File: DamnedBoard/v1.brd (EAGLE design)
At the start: 49.3 x 16.5 mm, 20 parts, among them J1 CORTEX_DEBUG_SMD, J2 GND, U1 EFM32ZG108, U2 MAX44009EDT+T21-0490D-M

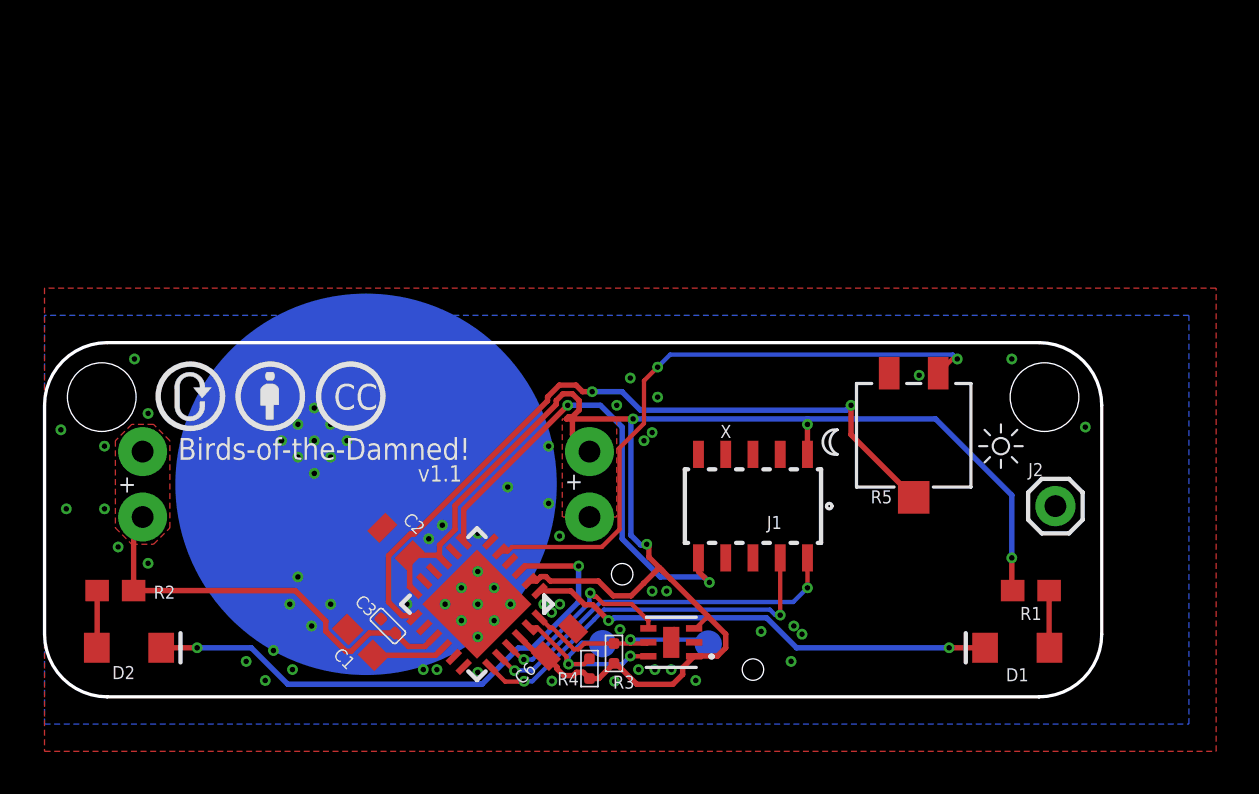
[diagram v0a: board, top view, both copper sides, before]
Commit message: Adding scheatic png
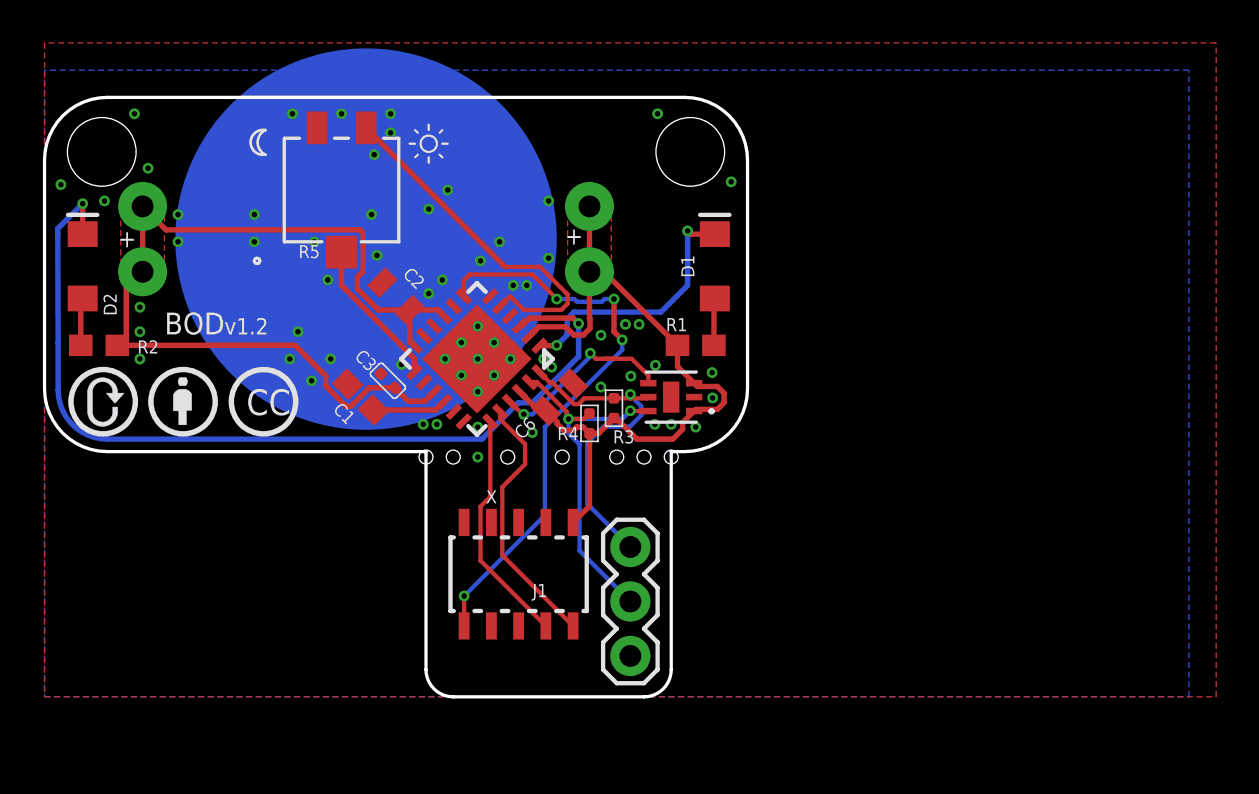
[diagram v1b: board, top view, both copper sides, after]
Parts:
- removed TP1, TP2: TEST-POINT3X5, SparkFun-Connectors:PAD.03X.05
- J2: value GND -> debug; device SparkFun-Connectors:1X01 -> SparkFun-Connectors:1X03
- moved R5 29.0 mm to (13.8, 23.6)
- moved D1 22.7 mm to (31.2, 20.1), turned to 90 degrees
- moved J2 19.9 mm to (27.3, 6.99), turned to 270 degrees
- moved R1 19.4 mm to (30.4, 16.4)
- moved D2 17.9 mm to (1.78, 20.1), turned to 90 degrees
- moved U$2 14.0 mm to (30.6, 11.9)
- moved R2 11.5 mm to (2.54, 16.4)
- moved C1 11.4 mm to (14.7, 14.0)
- moved C2 11.4 mm to (16.4, 18.7)
- moved C3 11.4 mm to (16.0, 14.7)
- moved C6 11.4 mm to (24.0, 14.0)
- moved G1 11.4 mm to (25.4, 22.9)
- moved R3 11.4 mm to (25.4, 12.7)
- moved R4 11.4 mm to (26.5, 13.5)
- moved U1 11.4 mm to (23.7, 15.7)
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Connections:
- net SCL: now also J2.1; no longer TP2.P$1
- net SDA: now also J2.2; no longer TP1.P$1
- net VSS: now also J2.3; no longer J2.1
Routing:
- net ADJ: track 34.7 -> 7.00 mm, vias 2 -> 0
- net VCC: track 100.7 -> 79.9 mm, vias 4 -> 0
- net EYE_R: track 26.3 -> 42.0 mm
- net ADJ_PWR: track 29.7 -> 16.8 mm, vias 2 -> 0
- net EYE_L: track 22.0 -> 12.4 mm
- net SDA: track 9.92 -> 17.4 mm
- net SWDCLK: track 18.0 -> 11.0 mm, vias 2 -> 0
- net SCL: track 9.89 -> 15.9 mm
- net SWDIO: track 17.6 -> 12.3 mm, vias 2 -> 0
- net NRESET: track 22.8 -> 26.9 mm, vias 2 -> 4
- net VSS: vias 69 -> 64
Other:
- board size 49.3 x 16.5 mm -> 32.8 x 27.9 mm
- board text added: "BOD"
- board text added: "v1.2"
- board text removed: "Birds-of-the-Damned!"
- board text removed: "v1.1"
